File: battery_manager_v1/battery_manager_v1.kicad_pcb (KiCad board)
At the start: 2 copper layers, 72.1 x 33 mm, 9 parts, among them U1 LT1761-SD, U2 LT1761-SD

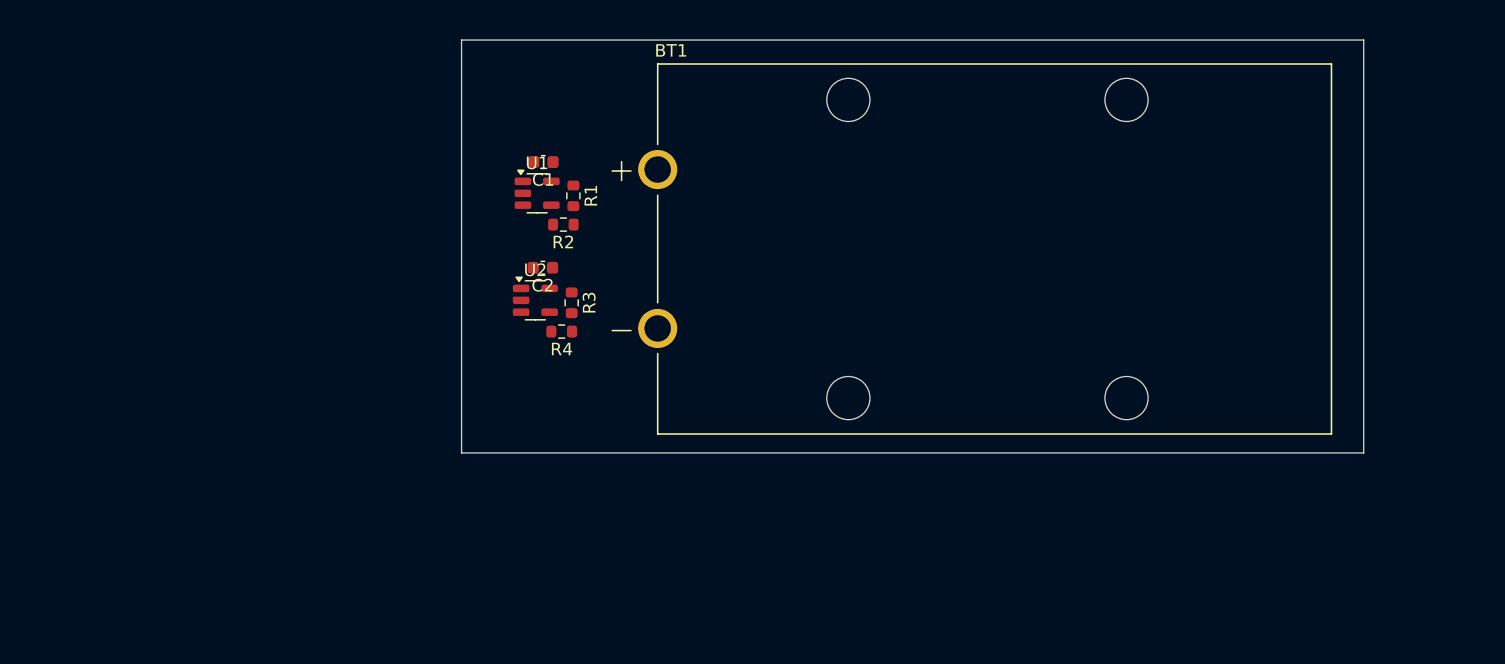
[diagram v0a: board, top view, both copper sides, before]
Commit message: V1 Final Before Update to V2
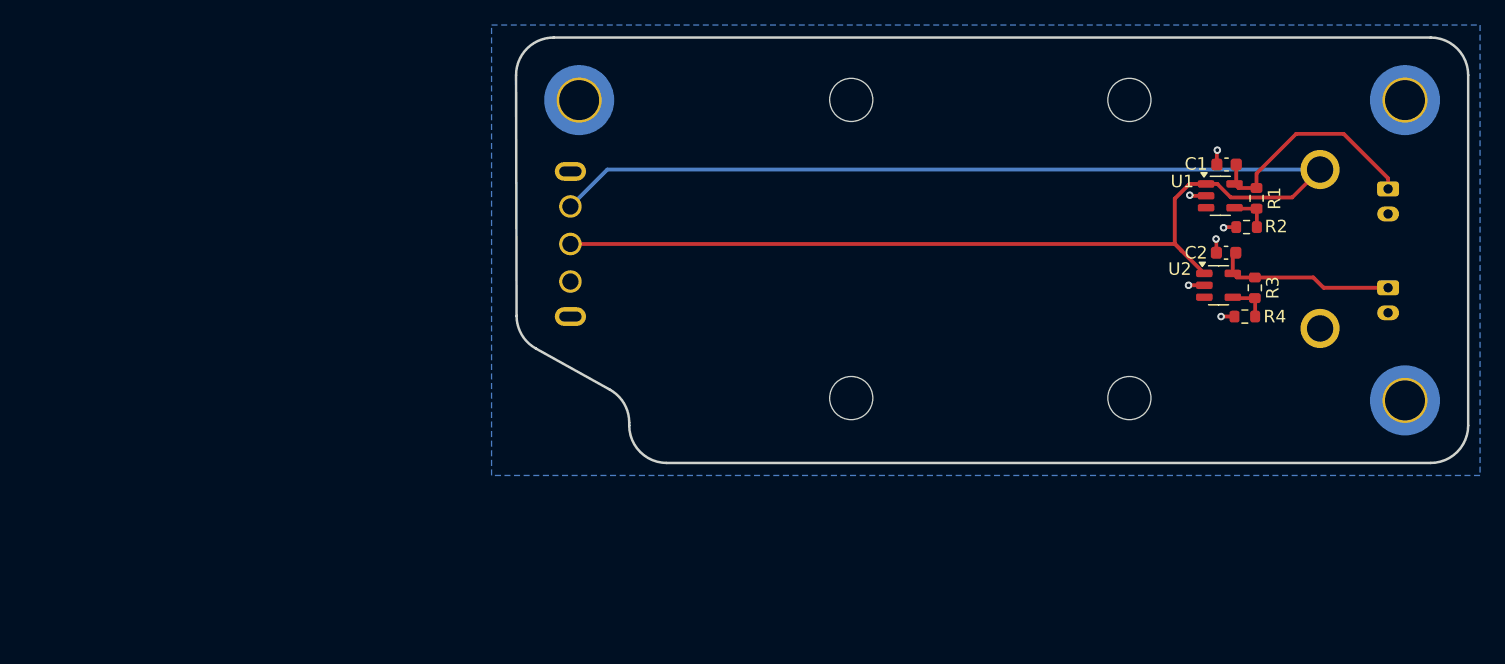
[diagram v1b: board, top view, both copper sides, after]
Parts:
- added H1: MountingHole_Pad, MountingHole:MountingHole_3.2mm_M3_DIN965_Pad_TopOnly, B.Cu at (68.0, 38.0)
- added H2: MountingHole_Pad, MountingHole:MountingHole_3.2mm_M3_DIN965_Pad_TopOnly, B.Cu at (134.0, 62.0)
- added H3: MountingHole_Pad, MountingHole:MountingHole_3.2mm_M3_DIN965_Pad_TopOnly, B.Cu at (134.0, 38.0)
- added J1: Conn_01x02, Connector_JST:JST_PH_S2B-PH-K_1x02_P2.00mm_Horizontal, B.Cu at (132.7, 53.0)
- added J2: Conn_01x02, Connector_JST:JST_PH_S2B-PH-K_1x02_P2.00mm_Horizontal, B.Cu at (132.7, 45.1)
- added SW1: SS-12F44-G5, LCSC Parts:SW-TH_SS-12F44-G5, B.Cu at (67.3, 49.5)
- BT1: footprint Battery Holder (Horizontal):BAT_1294 -> LCSC Parts:BAT_1294; moved to B.Cu
- moved C2 54.6 mm to (119.7, 50.2)
- moved R4 54.6 mm to (121.2, 55.3)
- moved R3 54.6 mm to (122.0, 53.0)
- moved U2 54.6 mm to (119.1, 52.8)
- moved R1 54.6 mm to (122.1, 45.9)
- moved R2 54.6 mm to (121.3, 48.1)
- moved C1 54.6 mm to (119.7, 43.1)
- moved U1 54.6 mm to (119.2, 45.6)
- moved BT1 0.91 mm to (100.3, 49.9), turned to 180 degrees
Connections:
- BT1 pad P: Net-(U1-VIN) -> Net-(BT1-PadP)
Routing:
- net Net-(U1-VIN): track 0.00 -> 69.5 mm
- net Net-(BT1-PadP): track 0.00 -> 61.1 mm
- net +5V: track 0.00 -> 18.8 mm
- net +8V: track 0.00 -> 14.6 mm
- net GND: track 0.00 -> 6.97 mm, vias 0 -> 6
- net Net-(U2-ADJ): track 0.00 -> 3.28 mm
- net Net-(U1-ADJ): track 0.00 -> 3.28 mm
- added copper zone on B.Cu, net GND
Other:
- board size 72.1 x 33 mm -> 76.1 x 34 mm

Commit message: Updates and first creation of gerbers
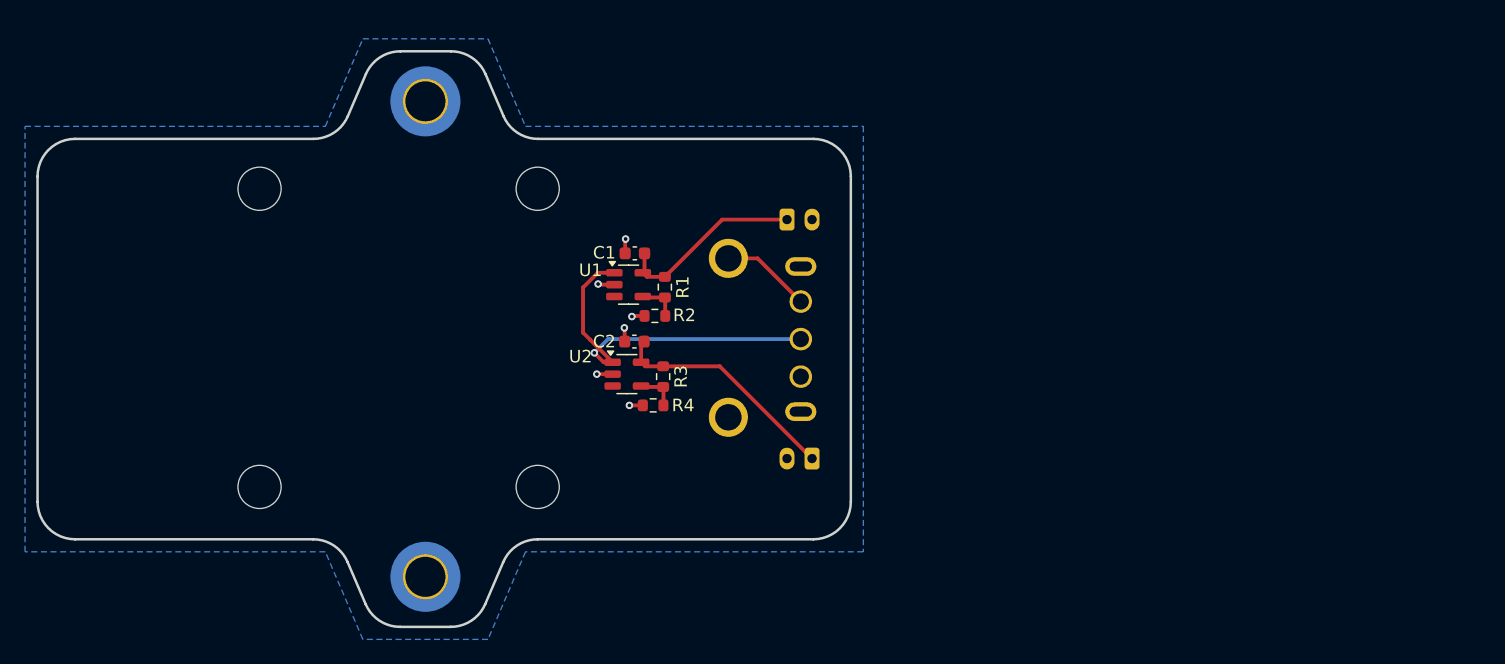
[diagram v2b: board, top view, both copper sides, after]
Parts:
- removed H3: MountingHole_Pad, MountingHole:MountingHole_3.2mm_M3_DIN965_Pad_TopOnly
- R1: value R_US -> 40.9k
- R2, R4: value R_US -> 10k
- R3: value R_US -> 65.5k
- moved H2 79.5 mm to (55.7, 76.1)
- moved J2 48.1 mm to (84.6, 47.5), turned to 0 degrees
- moved J1 48.0 mm to (86.6, 66.7), turned to 180 degrees
- moved BT1 47.8 mm to (53.0, 57.0)
- moved R1 47.8 mm to (74.8, 53.0)
- moved R2 47.8 mm to (74.0, 55.2)
- moved R3 47.8 mm to (74.7, 60.1)
- moved R4 47.8 mm to (73.9, 62.4)
- moved C2 47.8 mm to (72.4, 57.3)
- moved C1 47.8 mm to (72.4, 50.2)
- moved U1 47.8 mm to (71.9, 52.8)
- moved U2 47.8 mm to (71.8, 59.9)
- moved SW1 19.9 mm to (85.7, 57.1)
- moved H1 12.3 mm to (55.7, 38.1)
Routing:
- net Net-(BT1-PadP): track 61.1 -> 7.22 mm
- net Net-(U1-VIN): track 69.5 -> 28.7 mm, vias 0 -> 1
- net +8V: track 14.6 -> 18.6 mm
- net +5V: track 18.8 -> 15.2 mm
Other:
- board size 76.1 x 34 mm -> 65 x 46 mm
- board text added: "FR-4"
- board text added: "GND Plane"
- board text added: "Signal, SMD Fab"
- board text added: "Stackup:"
